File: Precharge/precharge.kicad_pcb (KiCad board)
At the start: 2 copper layers, 64.8 x 65.5 mm, 32 parts, among them J1 AIR_CONN, J2 TSAL_CONN_AIR, J3 TSAL_CONN_LV, J4 LV_CONN, J5 HV_CONN, J6 CAP_CONN, K1 IMB06IGR, Q1 AM2328NE, Q2 SQ2362, Q3 SQ2362, U1 ACPL-C87A-500E, U2 ACPL-C87A-500E, U3 MC34074ADR2G

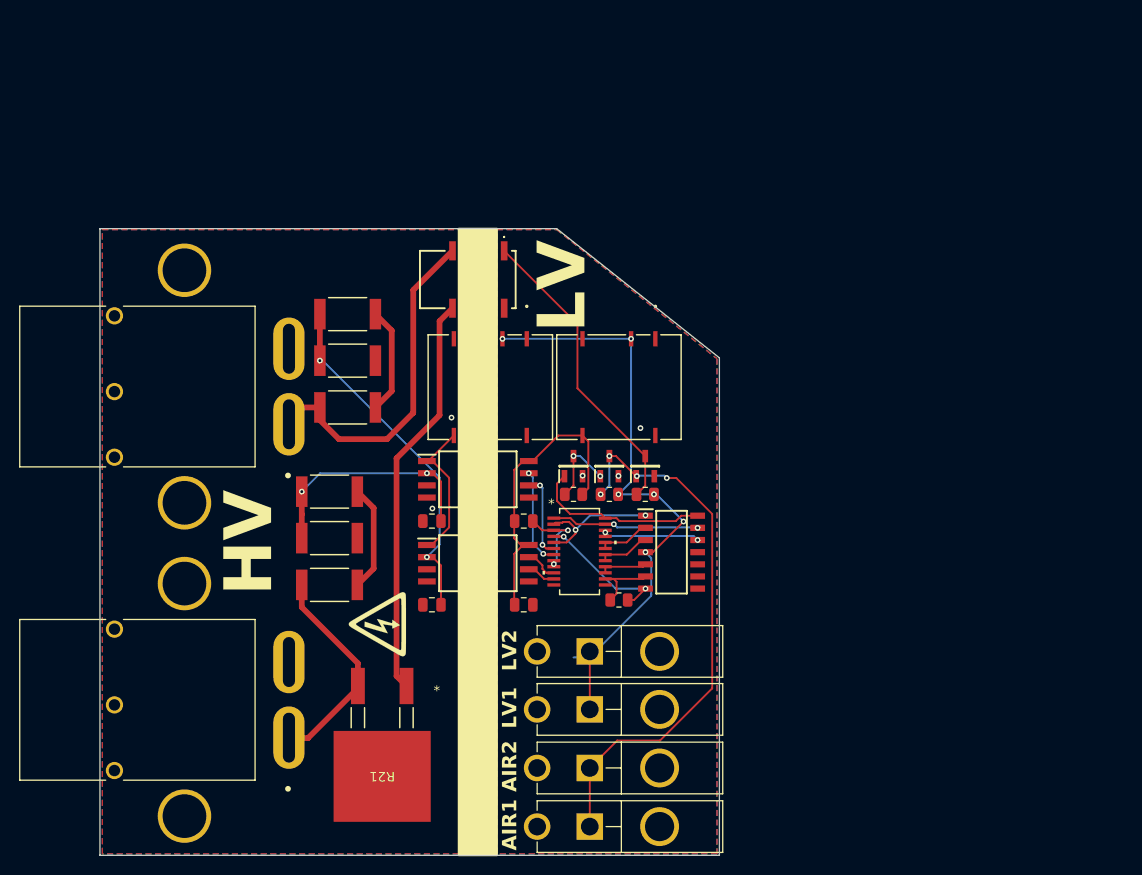
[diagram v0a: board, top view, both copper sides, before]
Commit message: Add files via upload
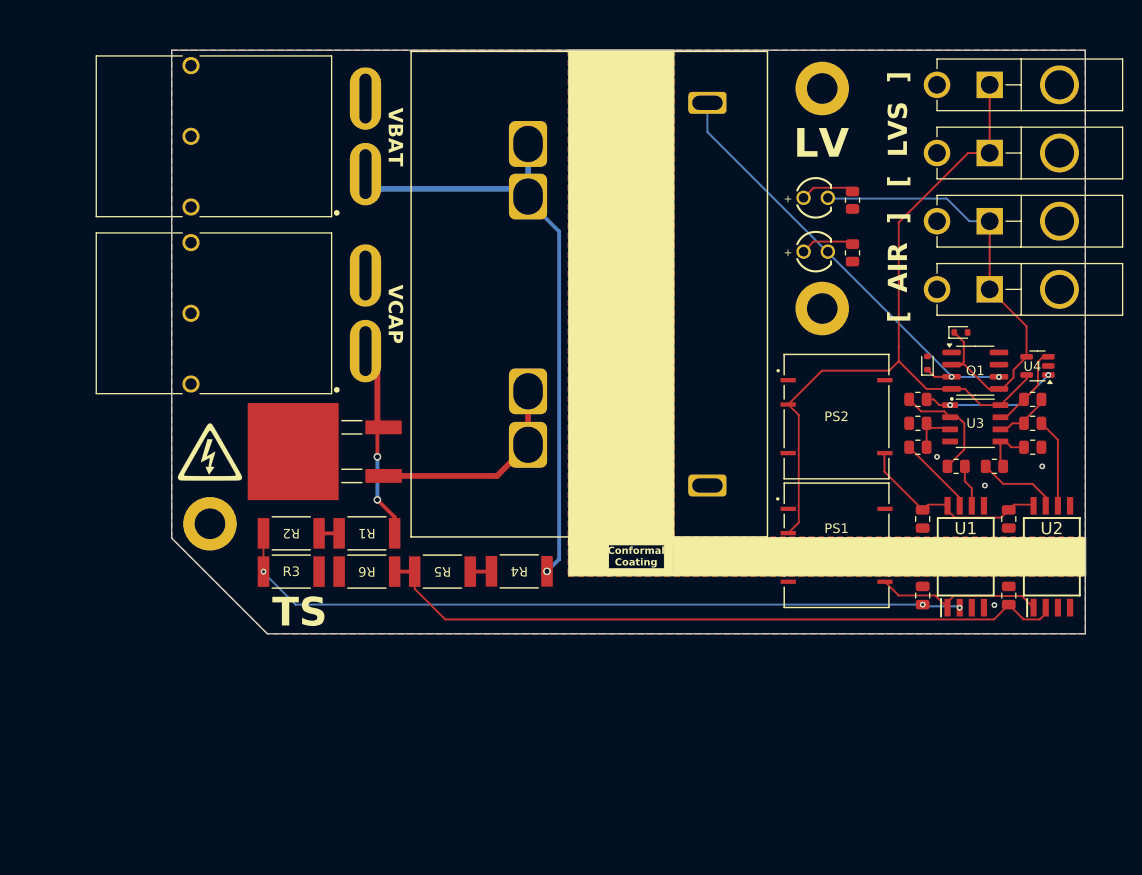
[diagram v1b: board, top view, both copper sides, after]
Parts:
- removed the G*** at (137.5, 129.0)
- removed Q2, Q3: SQ2362, customFootprints:SOT95P237X112-3N
- removed R19, R20, R22: 1K, Resistor_SMD:R_0805_2012Metric
- removed R21: 15K, customFootprints:PWR263S-35-1002F_BRN
- removed RN10K1: 10K, customFootprints:GULLWING24_VIS
- added D1: 1N4448X-TP, Diode_SMD:D_SOD-523, F.Cu at (195.0, 101.7)
- added D2: 151031VS06000, customFootprints:WL-TMRC_3MM, F.Cu at (183.3, 84.4)
- added D3: 151031SS06000, customFootprints:WL-TMRC_3MM, F.Cu at (183.3, 90.1)
- added D4: 1N4448X-TP, Diode_SMD:D_SOD-523, F.Cu at (198.5, 98.5)
- added G***: LOGO, customFootprints:electric-shock-symbol, F.Cu at (120.0, 111.0)
- added G***: LOGO, customFootprints:electric-shock-symbol, B.Cu at (120.0, 111.0)
- added R10: 10K, Resistor_SMD:R_0805_2012Metric, F.Cu at (198.0, 112.5)
- added R11: 10K, Resistor_SMD:R_0805_2012Metric, F.Cu at (194.0, 108.0)
- added R12: 10K, Resistor_SMD:R_0805_2012Metric, F.Cu at (194.0, 105.5)
- added R13: 10K, Resistor_SMD:R_0805_2012Metric, F.Cu at (202.0, 112.5)
- added R15: 10K, Resistor_SMD:R_0805_2012Metric, F.Cu at (206.0, 110.5)
- added R16: 600, Resistor_SMD:R_0805_2012Metric, F.Cu at (187.2, 84.7)
- added R17: 600, Resistor_SMD:R_0805_2012Metric, F.Cu at (187.2, 90.2)
- added R7: 15K, customFootprints:PWR263S-35-1002F_BRN, F.Cu at (128.7, 111.0)
- added R8: 9K7, Resistor_SMD:R_0805_2012Metric, F.Cu at (206.0, 105.5)
- added R9: 10K, Resistor_SMD:R_0805_2012Metric, F.Cu at (194.0, 110.5)
- added REF**: MountingHole_3.2mm_M3_DIN965_Pad, MountingHole:MountingHole_3.2mm_M3_DIN965_Pad, F.Cu at (184.0, 96.0)
- added REF**: MountingHole_3.2mm_M3_DIN965_Pad, MountingHole:MountingHole_3.2mm_M3_DIN965_Pad, F.Cu at (120.0, 118.5)
- added REF**: MountingHole_3.2mm_M3_DIN965_Pad, MountingHole:MountingHole_3.2mm_M3_DIN965_Pad, F.Cu at (184.0, 73.0)
- added U4: TL331, Package_TO_SOT_SMD:SOT-23-5, F.Cu at (206.5, 102.0)
- J1: value AIR_CONN -> CONN_AIR
- J4: value LV_CONN -> CONN_LV
- J5: value HV_CONN -> CONN_HV
- J6: value CAP_CONN -> CONN_CAP
- K1: value IMB06IGR -> 12V; footprint customFootprints:IMB03IGR -> customFootprints:RELAY_G9KB-1A_OMR
- Q1: value AM2328NE -> SI1539CDL-T1-GE3; footprint customFootprints:SOT95P237X112-3N -> Package_SO:SOIC-8_3.9x4.9mm_P1.27mm
- R1, R4: value 187K -> 124K
- R14: value 9K7 -> 10K
- R2, R5: value 11K -> 110K
- U3: value MC34074ADR2G -> MC33072DR2G; footprint customFootprints:SOIC127P600X175-14N -> customFootprints:SOIC127P600X175-8N
- moved J4 72.5 mm to (201.5, 72.6)
- moved J3 71.6 mm to (201.5, 79.7)
- moved J2 70.8 mm to (201.5, 86.9)
- moved J1 70.0 mm to (201.5, 94.0)
- moved C6 60.3 mm to (203.5, 126.0), turned to 90 degrees
- moved U2 60.0 mm to (208.0, 122.0), turned to 90 degrees
- moved C5 51.9 mm to (194.5, 126.0), turned to 90 degrees
- moved U1 51.6 mm to (199.0, 122.0), turned to 90 degrees
- moved C4 50.7 mm to (203.5, 118.0), turned to 90 degrees
- moved R14 47.0 mm to (206.0, 108.0), turned to 180 degrees
- moved J6 45.5 mm to (118.0, 96.5)
- moved Q1 43.2 mm to (200.0, 102.5), turned to 0 degrees
- moved C3 42.7 mm to (194.5, 118.0), turned to 90 degrees
- moved PS1 39.8 mm to (185.5, 120.8), turned to 0 degrees
- moved U3 34.5 mm to (200.0, 108.0)
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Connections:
- net VBAT_0.5% renamed Net-(U2-IN)
- net VCAP_0.5% renamed Net-(U1-IN)
- C3 pad 1: AIR- -> LVGND
- C4 pad 1: AIR- -> LVGND
- J1 pad 2: AIR- -> LVGND
- J2 pad 2: AIR- -> LVGND
- J3 pad 2: AIR- -> LVGND
- J4 pad 2: AIR- -> LVGND
- K1 pad 1: CHARGE_EN -> LVGND
- K1 pad 3: VBAT -> Net-(K1-Pad3)
- K1 pad 6: Net-(K1-Pad6) -> VBAT
- PS1 pad 1: AIR- -> LVGND
- PS2 pad 1: AIR- -> LVGND
- PS2 pad 4: AIR- -> LVGND
- Q1 pad 1: Net-(Q1-G) -> LVGND
- Q1 pad 2: AIR- -> AIR+
- Q1 pad 3: Net-(Q1-D) -> CHARGE-EN
- R14 pad 1: Net-(U3B--) -> Net-(U2-OUT-)
- R14 pad 2: Net-(R14-Pad2) -> Net-(U3B--)
- U1 pad 5: AIR- -> LVGND
- U2 pad 5: AIR- -> LVGND
- U3 pad 4: +12V -> LVGND
- U3 pad 7: Net-(R14-Pad2) -> Net-(U4-+)
- U3 pad 8: (no net) -> +12V
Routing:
- net Net-(U1-IN): track 24.7 -> 78.5 mm, vias 2 -> 3
- net CHARGE-EN: track 0.00 -> 47.4 mm, vias 0 -> 2
- net Net-(K1-Pad6): track 42.3 -> 0.00 mm
- net Net-(U2-IN): track 37.9 -> 73.4 mm, vias 2 -> 0
- net CHARGE_EN: track 31.9 -> 0.00 mm
- net VBAT: track 35.0 -> 64.2 mm, vias 0 -> 1
- net Net-(K1-Pad3): track 0.00 -> 23.6 mm
- net Net-(Q1-G): track 18.7 -> 0.00 mm
- net Net-(U3C--): track 15.5 -> 0.00 mm, vias 2 -> 0
- net Net-(R14-Pad2): track 14.2 -> 0.00 mm, vias 2 -> 0
- net +12V: track 64.9 -> 78.8 mm, vias 6 -> 0
- net +5V_LV: track 31.5 -> 20.9 mm
- net Net-(U3C-+): track 10.2 -> 0.00 mm, vias 2 -> 0
- net AIR-: track 9.41 -> 0.00 mm, vias 5 -> 0
- net Net-(R1-Pad2): track 11.2 -> 2.10 mm
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- added copper zone on B.Cu, net LVGND
- added copper zone on F.Cu, net LVGND
- removed copper zone on B.Cu, net AIR-
- removed copper zone on F.Cu, net AIR-
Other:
- board size 64.8 x 65.5 mm -> 95.5 x 61 mm
- board text added: "Conformal Coating"
- board text added: "TS"
- board text added: "VBAT"
- board text added: "VCAP"
- board text added: "[ AIR ]"
- board text added: "[ LVS ]"
- board text removed: "AIR1"
- board text removed: "AIR2"
- board text removed: "HV"
- board text removed: "LV1"
- board text removed: "LV2"
